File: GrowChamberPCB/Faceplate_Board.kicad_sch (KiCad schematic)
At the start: 56 parts, among them J11 Conn_01x26_Pin, J12 Fogger Fill Solenoid, J13 Drain Solenoid, J14 Glycol Solenoid, J15 Fogger Disc, J16 Fogger Float, J17 Drain Level, J18 Heater Fans Con, J19 Soil Moisture 2, J20 Soil Moisture 3, J21 Soil Moisture 1, J22 Fan Connector, J23 SCD30 Connector, J24 Conn_01x02_Pin, J4 Glycol Fans, J5 Circ Fans, J6 UART, J8 Screw_Terminal_01x03, J9 Water Solenoid, SW1 BootMode_Switch, SW2 ResetButton_External, U7 PCA9555PW,118

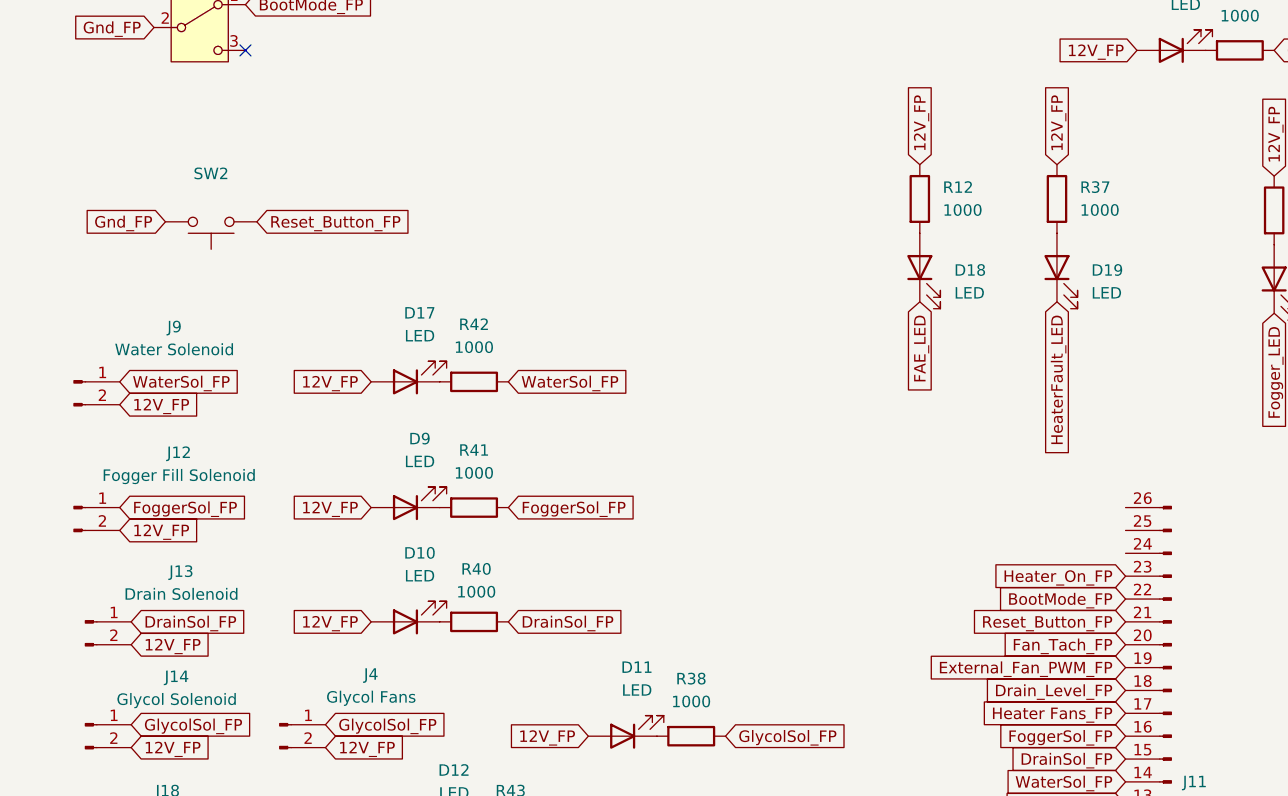
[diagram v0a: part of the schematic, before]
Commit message: working on stuff
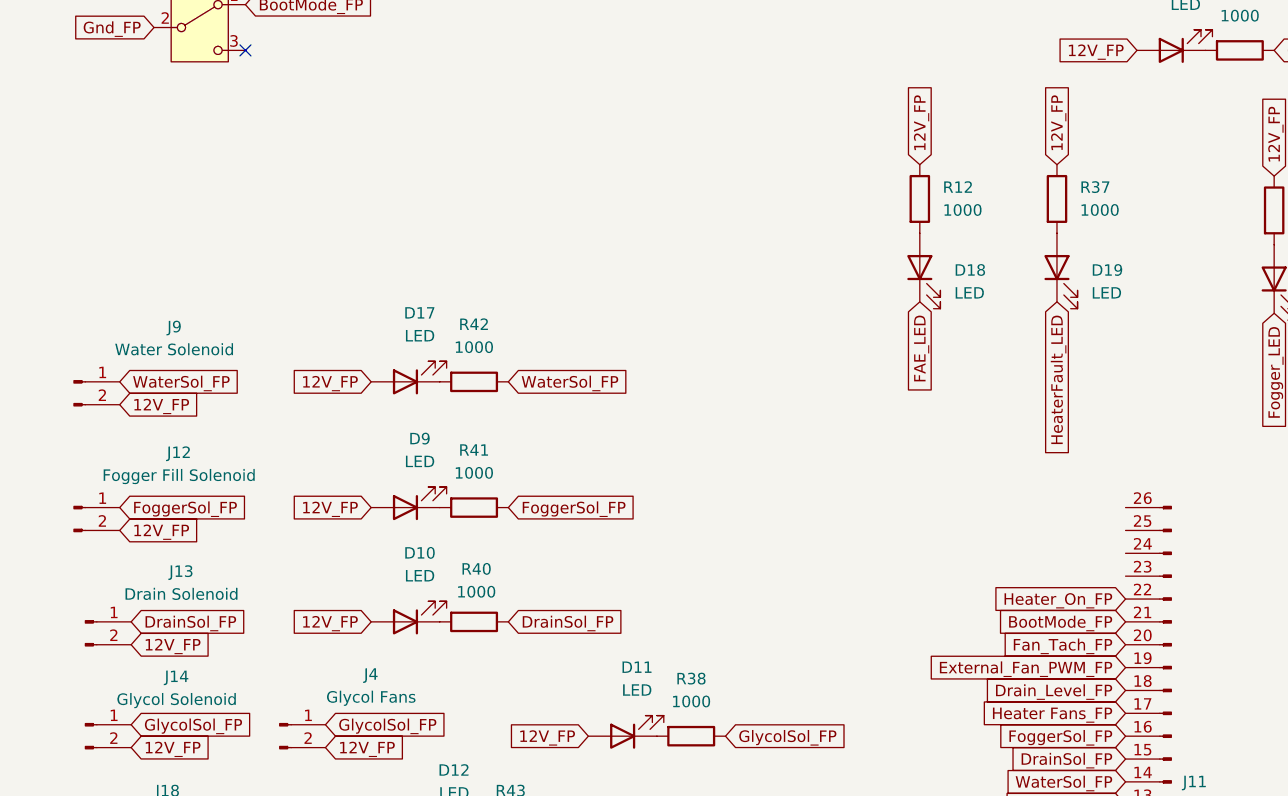
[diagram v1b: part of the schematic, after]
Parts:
- removed SW2: ResetButton_External, symbol Switch:SW_Push
- J13, J14, J17, J18: footprint Connector_Molex:Molex_KK-254_AE-6410-03A_1x03_P2.54mm_Vertical -> Connector_Molex:Molex_KK-254_AE-6410-02A_1x02_P2.54mm_Vertical
- J22: footprint Connector_Molex:Molex_KK-254_AE-6410-03A_1x03_P2.54mm_Vertical -> Connector_Molex:Molex_KK-254_AE-6410-04A_1x04_P2.54mm_Vertical
- SW1: footprint (none) -> Button_Switch_THT:SW_Slide_SPDT_Straight_CK_OS102011MS2Q; MFG Part Number (none) -> SS12D07VG4; Manufacturer (none) -> HanElectricity; Package (none) -> Plugin-5P,8.7x4.4mm
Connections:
- net Reset_Button_FP is gone; now on net BootMode_FP: J11.21 (Pin_21)
- net BootMode_FP: no longer J11.22 (Pin_22)
- net Heater_On_FP: now also J11.22 (Pin_22); no longer J11.23 (Pin_23)
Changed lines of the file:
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@@
 		)
 	)
-	(global_label "Reset_Button_FP"
-		(shape input)
-		(at 36.83 59.69 0)
-		(fields_autoplaced yes)
-		(effects
-			(font
-				(size 1.27 1.27)
-			)
-			(justify left)
-		)
-		(property "Intersheetrefs" "${INTERSHEET_REFS}"
-			(at 55.4784 59.69 0)
-			(effects
-				(font
-					(size 1.27 1.27)
-				)
-				(justify left)
-				(hide yes)
-			)
-		)
-	)
 	(global_label "Drain_Level_FP"
 		(shape input)
@@
 		)
 	)
-	(global_label "Reset_Button_FP"
-		(shape input)
-		(at 133.35 104.14 180)
-		(fields_autoplaced yes)
-		(effects
-			(font
-				(size 1.27 1.27)
-			)
-			(justify right)
-		)
-		(property "Intersheetrefs" "${INTERSHEET_REFS}"
-			(at 114.7016 104.14 0)
-			(effects
-				(font
-					(size 1.27 1.27)
-				)
-				(justify right)
-				(hide yes)
-			)
-		)
-	)
-	(global_label "Gnd_FP"
-		(shape input)
-		(at 26.67 59.69 180)
-		(fields_autoplaced yes)
-		(effects
-			(font
-				(size 1.27 1.27)
-			)
-			(justify right)
-		)
-		(property "Intersheetrefs" "${INTERSHEET_REFS}"
-			(at 16.7906 59.69 0)
-			(effects
-				(font
-					(size 1.27 1.27)
-				)
-				(justify right)
-				(hide yes)
-			)
-		)
-	)
 	(global_label "LEDs_FP"
 		(shape input)
@@
 		)
 	)
-	(global_label "BootMode_FP"
+	(global_label "Heater_On_FP"
 		(shape input)
 		(at 133.35 101.6 180)
@@
 		)
 		(property "Intersheetrefs" "${INTERSHEET_REFS}"
-			(at 117.9069 101.6 0)
+			(at 117.4229 101.6 0)
 			(effects
 				(font
@@
 		)
 	)
+	(global_label "BootMode_FP"
+		(shape input)
+		(at 133.35 104.14 180)
+		(fields_autoplaced yes)
+		(effects
+			(font
+				(size 1.27 1.27)
+			)
+			(justify right)
+		)
+		(property "Intersheetrefs" "${INTERSHEET_REFS}"
+			(at 117.9069 104.14 0)
+			(effects
+				(font
+					(size 1.27 1.27)
+				)
+				(justify right)
+				(hide yes)
+			)
+		)
+	)
 	(global_label "12V_FP"
 		(shape input)
@@
 		)
 	)
-	(global_label "Heater_On_FP"
-		(shape input)
-		(at 133.35 99.06 180)
-		(fields_autoplaced yes)
-		(effects
-			(font
-				(size 1.27 1.27)
-			)
-			(justify right)
-		)
-		(property "Intersheetrefs" "${INTERSHEET_REFS}"
-			(at 117.4229 99.06 0)
-			(effects
-				(font
-					(size 1.27 1.27)
-				)
-				(justify right)
-				(hide yes)
-			)
-		)
-	)
 	(global_label "12V_FP"
 		(shape input)
@@
 			)
 		)
-		(property "Footprint" "Connector_Molex:Molex_KK-254_AE-6410-03A_1x03_P2.54mm_Vertical"
+		(property "Footprint" "Connector_Molex:Molex_KK-254_AE-6410-02A_1x02_P2.54mm_Vertical"
 			(at 17.78 104.14 0)
 			(effects
@@
 			)
 		)
-		(property "Footprint" ""
+		(property "Footprint" "Button_Switch_THT:SW_Slide_SPDT_Straight_CK_OS102011MS2Q"
 			(at 30.48 38.1 0)
 			(effects
@@
 			)
 		)
-		(property "Description" "Switch, single pole double throw"
+		(property "Description" "4.4mm 8.7mm 8.7mm Black PC Pin Rectangular Columnar SPDT Through Hole 插件-5P,8.7x4.4mm Slide Switches ROHS"
 			(at 30.48 38.1 0)
 			(effects
@@
 			)
 		)
-		(property "MFG Part Number" ""
+		(property "MFG Part Number" "SS12D07VG4"
+			(at 30.48 38.1 0)
+			(effects
+				(font
+					(size 1.27 1.27)
+				)
+				(hide yes)
+			)
+		)
+		(property "Manufacturer" "HanElectricity"
+			(at 30.48 38.1 0)
+			(effects
+				(font
+					(size 1.27 1.27)
+				)
+				(hide yes)
+			)
+		)
+		(property "Package" "Plugin-5P,8.7x4.4mm"
 			(at 30.48 38.1 0)
 			(effects
@@
 		)
 		(instances
-			(project ""
+			(project "GrowChamberPCB"
 				(path "/39371779-5336-4073-adec-fb32caf6a86f/b570075a-c3a2-42a6-b1ef-d9defe6d89ee"
 					(reference "SW1")
@@
 			)
 		)
-		(property "Footprint" "Connector_Molex:Molex_KK-254_AE-6410-03A_1x03_P2.54mm_Vertical"
+		(property "Footprint" "Connector_Molex:Molex_KK-254_AE-6410-02A_1x02_P2.54mm_Vertical"
 			(at 17.78 128.27 0)
 			(effects
@@
 			)
 		)
-		(property "Footprint" "Connector_Molex:Molex_KK-254_AE-6410-03A_1x03_P2.54mm_Vertical"
+		(property "Footprint" "Connector_Molex:Molex_KK-254_AE-6410-02A_1x02_P2.54mm_Vertical"
 			(at 17.78 115.57 0)
 			(effects
@@
 			)
 		)
-		(property "Footprint" "Connector_Molex:Molex_KK-254_AE-6410-03A_1x03_P2.54mm_Vertical"
+		(property "Footprint" "Connector_Molex:Molex_KK-254_AE-6410-02A_1x02_P2.54mm_Vertical"
 			(at 218.44 130.81 0)
 			(effects
@@
 			)
 		)
-		(property "Footprint" "Connector_Molex:Molex_KK-254_AE-6410-03A_1x03_P2.54mm_Vertical"
+		(property "Footprint" "Connector_Molex:Molex_KK-254_AE-6410-04A_1x04_P2.54mm_Vertical"
 			(at 43.18 180.34 0)
 			(effects
@@
 					(unit 1)
 				)
-			)
-		)
-	)
-	(symbol
-		(lib_id "Switch:SW_Push")
-		(at 31.75 59.69 180)
-		(unit 1)
-		(exclude_from_sim no)
-		(in_bom yes)
-		(on_board yes)
-		(dnp no)
-		(property "Reference" "SW2"
-			(at 31.75 54.356 0)
-			(effects
-				(font
-					(size 1.27 1.27)
-				)
-			)
-		)
-		(property "Value" "ResetButton_External"
-			(at 31.75 56.896 0)
-			(effects
-				(font
-					(size 1.27 1.27)
-				)
-				(hide yes)
-			)
-		)
-		(property "Footprint" ""
-			(at 31.75 64.77 0)
-			(effects
-				(font
-					(size 1.27 1.27)
-				)
-				(hide yes)
-			)
-		)
-		(property "Datasheet" "~"
-			(at 31.75 64.77 0)
-			(effects
-				(font
-					(size 1.27 1.27)
-				)
-				(hide yes)
-			)
-		)
-		(property "Description" "Push button switch, generic, two pins"
-			(at 31.75 59.69 0)
-			(effects
-				(font
-					(size 1.27 1.27)
-				)
-				(hide yes)
-			)
-		)
-		(property "MFG Part Number" ""
-			(at 31.75 59.69 0)
-			(effects
-				(font
-					(size 1.27 1.27)
-				)
-				(hide yes)
-			)
-		)
-		(property "Type (SMD/thru-hole, etc.)" ""
-			(at 31.75 59.69 0)
-			(effects
-				(font
-					(size 1.27 1.27)
-				)
-				(hide yes)
-			)
-		)
-		(property "Manufacturer" ""
-			(at 31.75 59.69 0)
-			(effects
-				(font
-					(size 1.27 1.27)
-				)
-				(hide yes)
-			)
-		)
-		(property "Package" ""
-			(at 31.75 59.69 0)
-			(effects
-				(font
-					(size 1.27 1.27)
-				)
-				(hide yes)
-			)
-		)
-		(pin "2"
-		)
-		(pin "1"
-		)
-		(instances
-			(project "GrowChamberPCB"
-				(path "/39371779-5336-4073-adec-fb32caf6a86f/b570075a-c3a2-42a6-b1ef-d9defe6d89ee"
-					(reference "SW2")
-					(unit 1)
-				)
